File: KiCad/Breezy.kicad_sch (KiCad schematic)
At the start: 9 parts, among them J1 Line Voltage Input 120VAC / 6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, J2 Line Voltage Output 120VAC / 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, K1 5V, Q1 2N3904

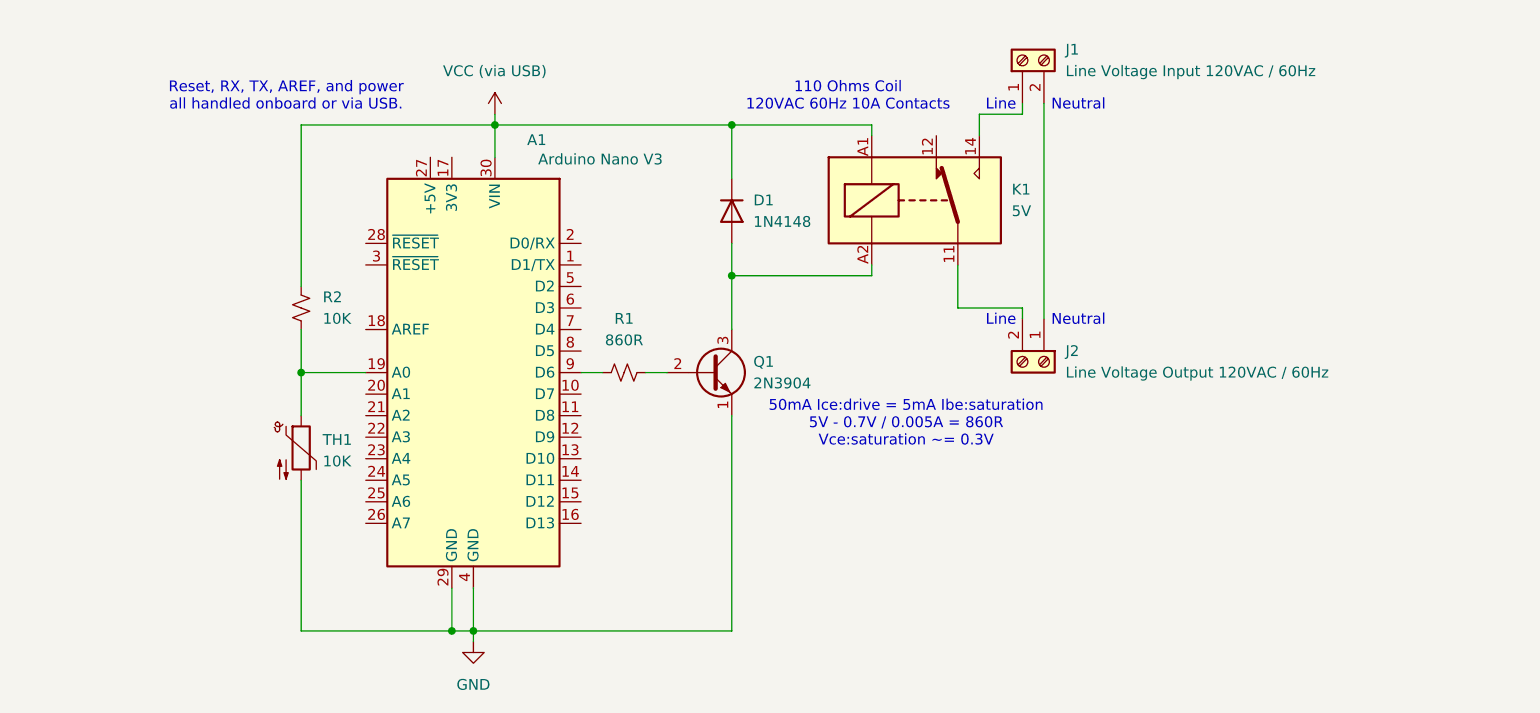
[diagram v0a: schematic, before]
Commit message: Update
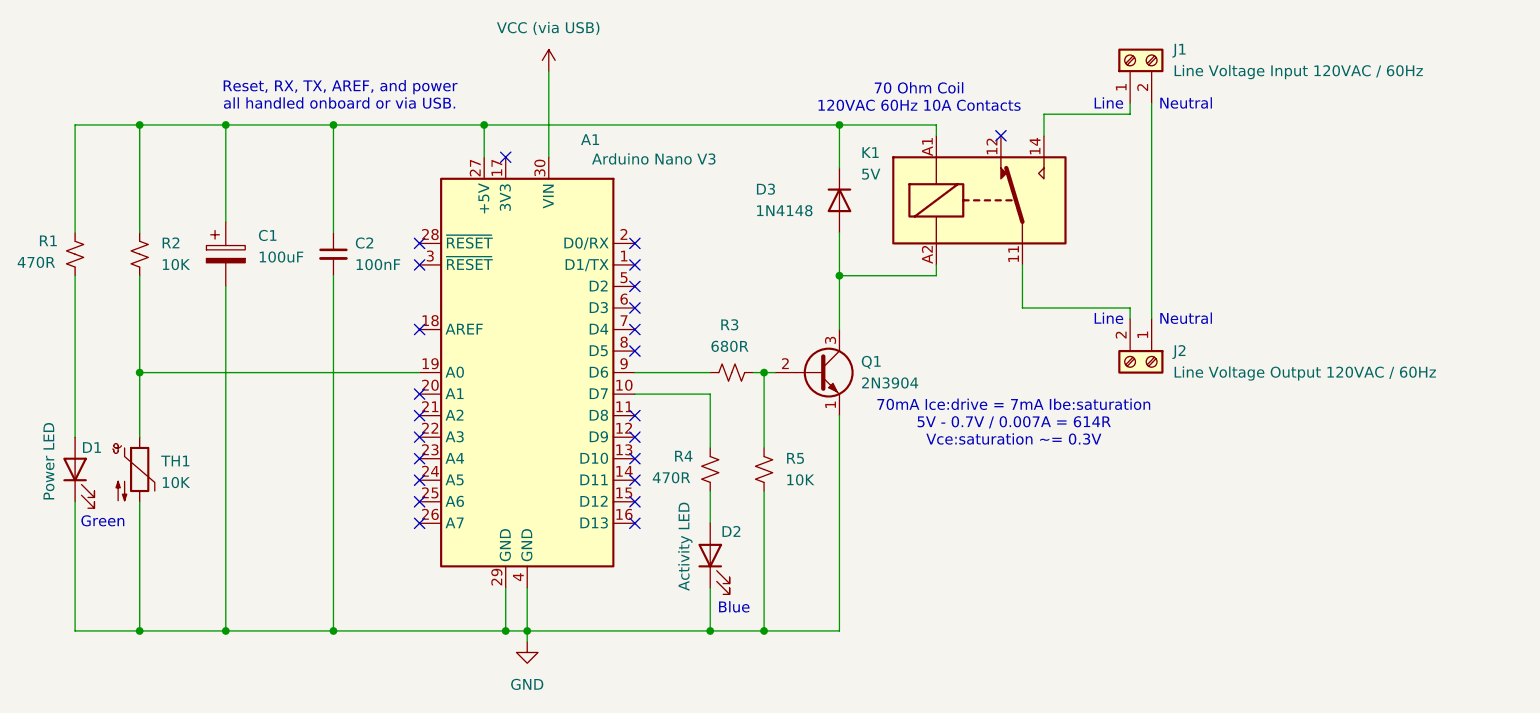
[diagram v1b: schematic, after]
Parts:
- added C1: 100uF, symbol Device:C_Polarized
- added C2: 100nF, symbol Device:C_Small
- added D1: Power LED, symbol Device:LED
- added D2: Activity LED, symbol Device:LED
- added R1, R4: 470R, symbol Device:R_Small_US
- added R5: 10K, symbol Device:R_Small_US
- R3: renamed from R1; value 860R -> 680R
- renumbered D1 to D3
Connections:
- net GND: now also C1.2, C2.2, D1.1 (K), D2.1 (K), R5.2
- net VCC (via USB): no longer D3.1 (K), K1.A1, R2.1
- net at Q1.2 (B), R3.1: now also R5.1
- net at A1.10 (D7): now also R4.1
- net at A1.27 (+5V): now also D3.1 (K), K1.A1, R2.1, C1.1, C2.1, R1.1
- new net: D2.2 (A), R4.2
- new net: D1.2 (A), R1.2
- no-connect marks 0 -> 24
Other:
- note added: "70 Ohm Coil 120VAC 60Hz 10A Contacts"
- note added: "70mA Ice:drive = 7mA Ibe:saturation 5V - 0.7V / 0.007A = 614R Vce:saturation ~= 0.3V"
- note added: "Blue"
- note added: "Green"
- note removed: "110 Ohms Coil 120VAC 60Hz 10A Contacts"
- note removed: "50mA Ice:drive = 5mA Ibe:saturation 5V - 0.7V / 0.005A = 860R Vce:saturation ~= 0.3V"
- moved on the sheet: A1, D3, J1, J2, K1, Q1, R2, R3, TH1
